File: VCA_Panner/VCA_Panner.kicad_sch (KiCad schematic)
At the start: 40 parts, among them J1 CV1, J2 Ch1_in, J3 Ch1_out, J4 CV2, J5 Ch2_in, J6 Ch2_out, SW1 SW_DPDT_x2, SW2 SW_DPDT_x2, U1 TL074, U2 AS3360, U3 TL072

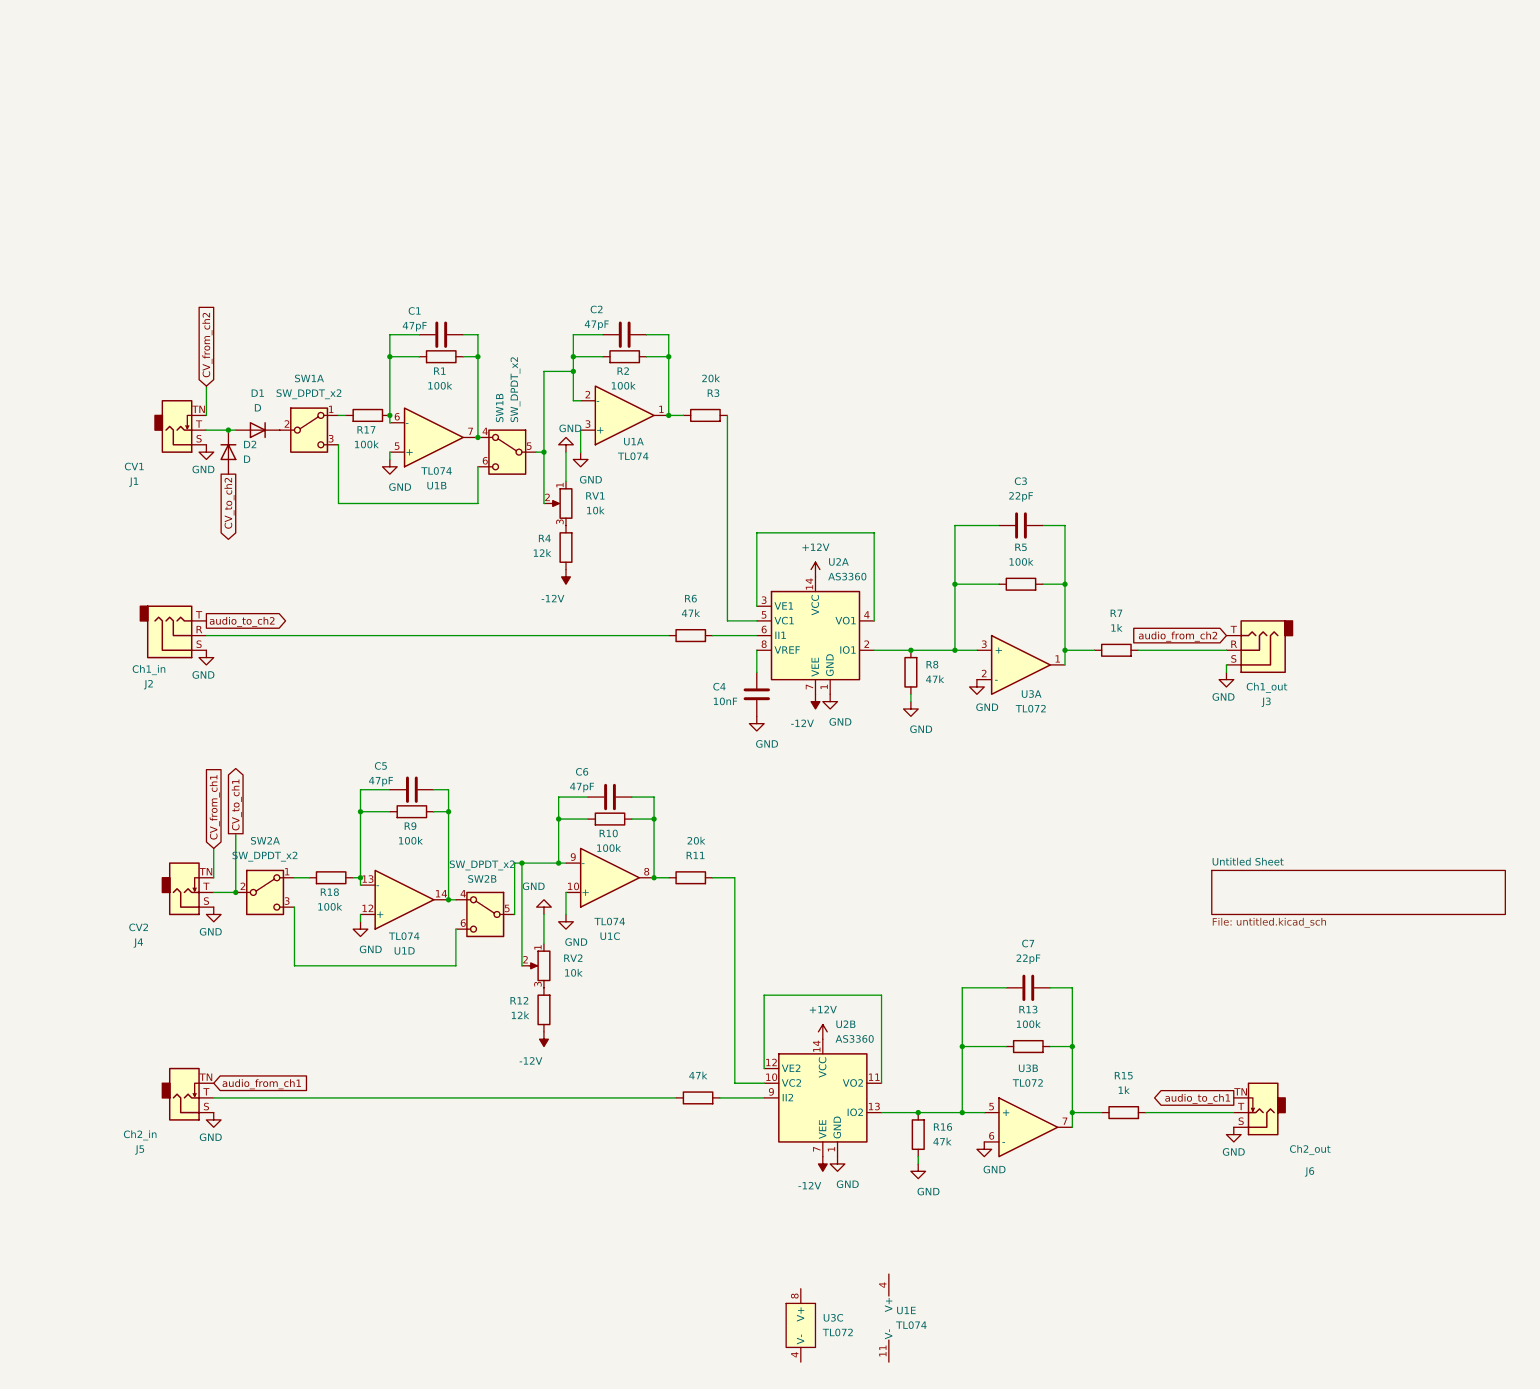
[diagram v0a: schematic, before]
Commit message: almost working
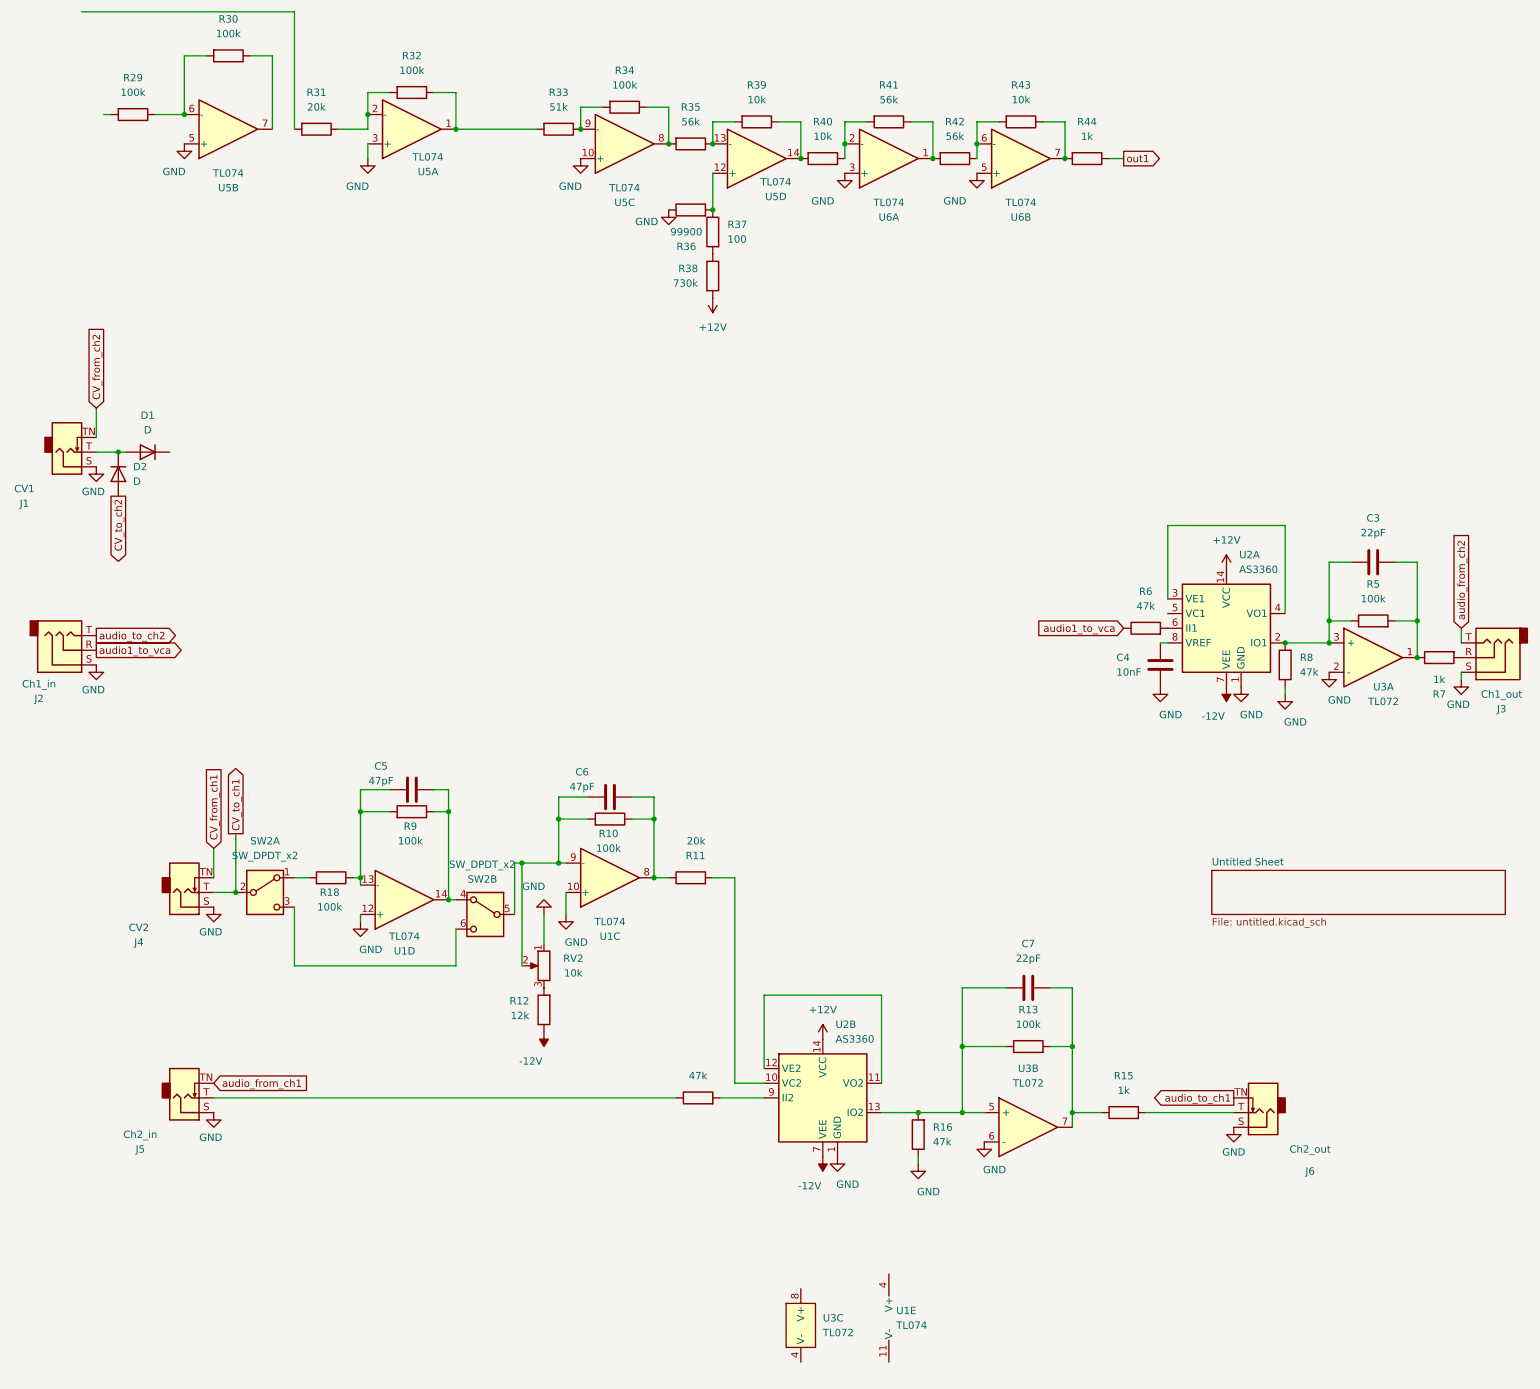
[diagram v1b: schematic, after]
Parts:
- removed C1, C2: 47pF, symbol Device:C
- removed R1, R17, R2: 100k, symbol Device:R
- removed R3: 20k, symbol Device:R
- removed R4: 12k, symbol Device:R
- removed RV1: 10k, symbol Device:R_Potentiometer
- removed SW1: SW_DPDT_x2, symbol Switch:SW_DPDT_x2
- removed unit 1 of U1
- removed unit 2 of U1
- added R29, R30, R32, R34: 100k, symbol Device:R
- added R31: 20k, symbol Device:R
- added R33: 51k, symbol Device:R
- added R35, R41, R42: 56k, symbol Device:R
- added R36: 99900, symbol Device:R
- added R37: 100, symbol Device:R
- added R38: 730k, symbol Device:R
- added R39, R40, R43: 10k, symbol Device:R
- added R44: 1k, symbol Device:R
- added U5, U6: TL074, symbol Amplifier_Operational:TL074
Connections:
- net +12V: now also R38.2
- net GND: now also R36.1, U5.10 (+), U5.3 (+), U5.5 (+), U6.3 (+), U6.5 (+)
- net audio1_to_vca: now reaches J2.R, R6.1
- new net: R32.1, R33.2, U5.1
- new net: R31.1, R32.2, U5.2 (-)
- new net: R36.2, R37.1, U5.12 (+)
- new net: R37.2, R38.1
- new net: R35.1, R39.2, U5.13 (-)
- new net: R39.1, R40.2, U5.14
- new net: R43.1, R44.2, U6.7
- new net: R42.1, R43.2, U6.6 (-)
- new net: R30.1, U5.7
- new net: R29.1, R30.2, U5.6 (-)
- new net: R33.1, R34.2, U5.9 (-)
- new net: R41.1, R42.2, U6.1
- new net: R40.1, R41.2, U6.2 (-)
- new net: R34.1, R35.2, U5.8
- new net out1: R44.1
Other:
- moved on the sheet: C3, C4, D1, D2, J1, J2, J3, R5, R6, R7, R8, U2A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

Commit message: finished schematic
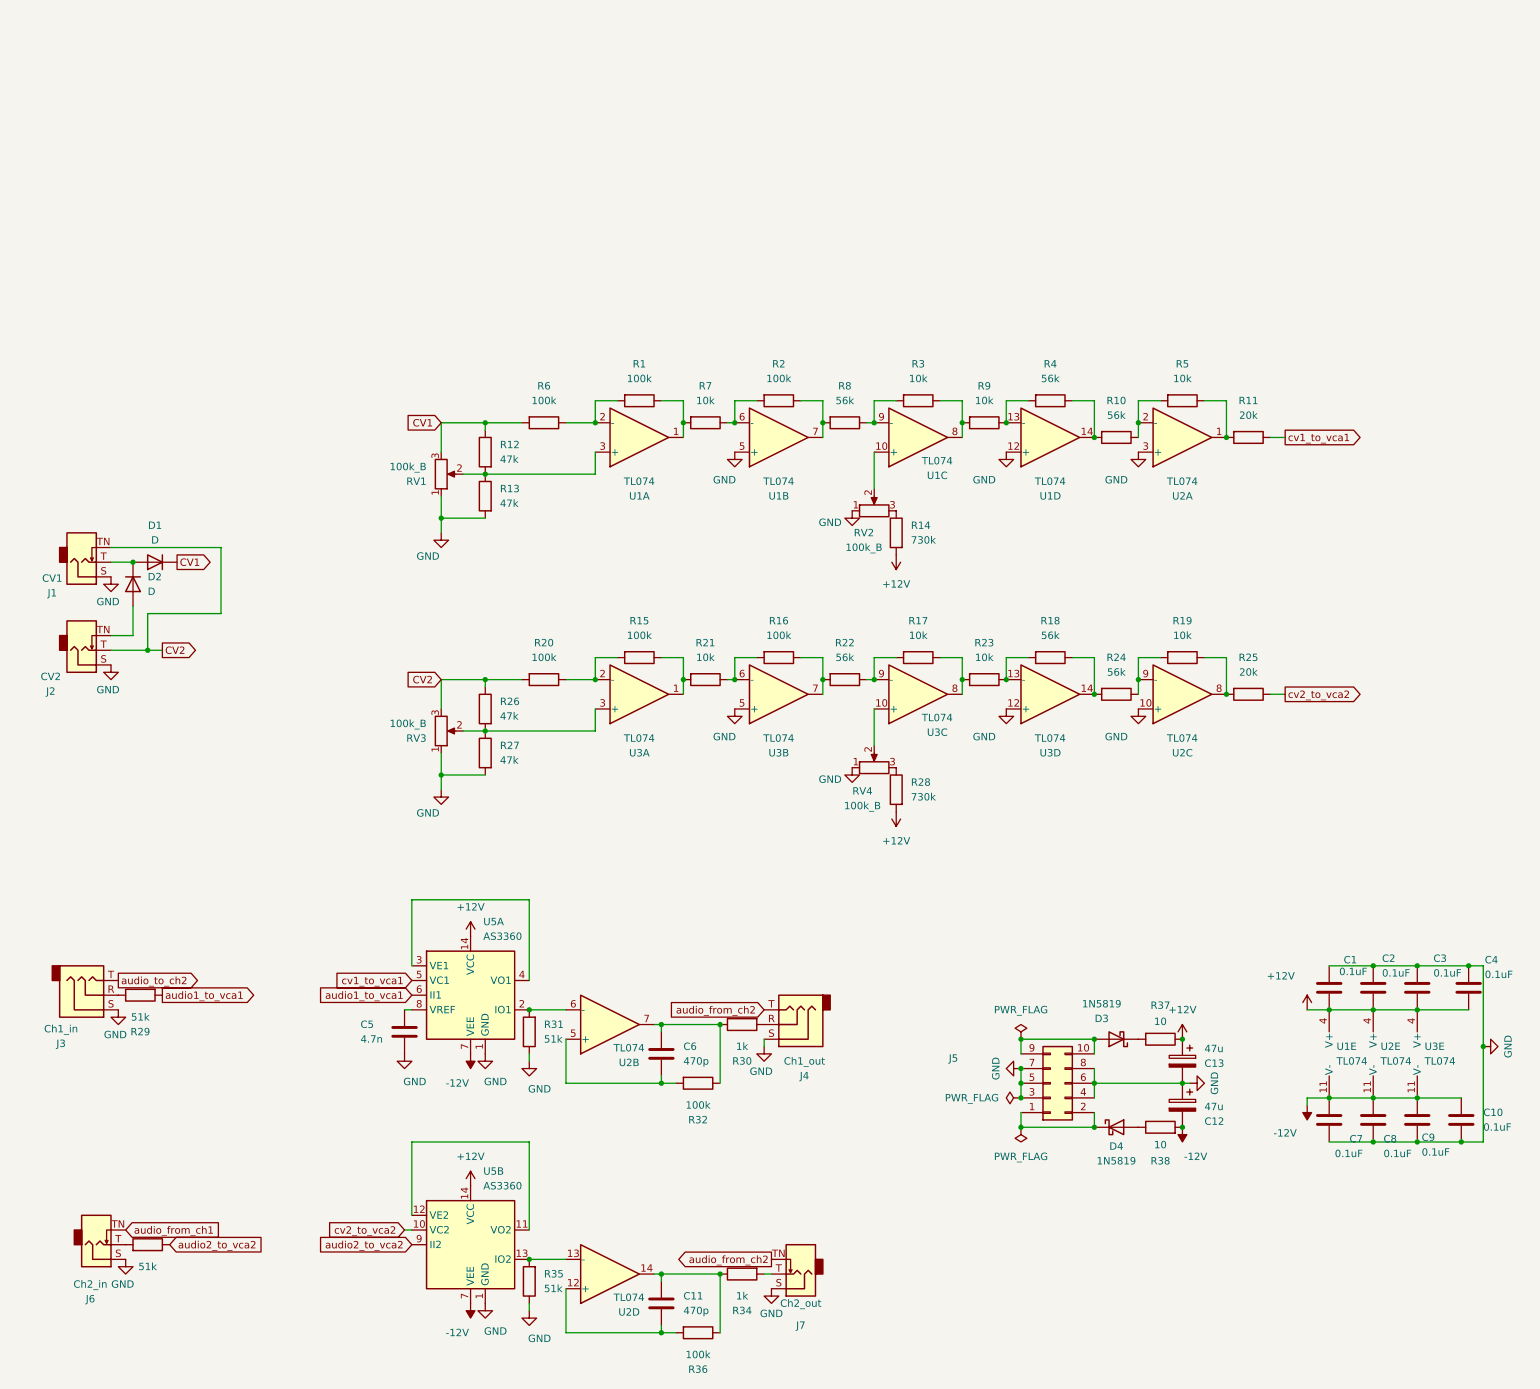
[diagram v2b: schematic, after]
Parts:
- removed C5: 47pF, symbol Device:C
- removed R30: 100k, symbol Device:R
- removed R31: 20k, symbol Device:R
- removed R39, R40, R43: 10k, symbol Device:R
- removed R41, R42: 56k, symbol Device:R
- removed R44: 1k, symbol Device:R
- removed SW2: SW_DPDT_x2, symbol Switch:SW_DPDT_x2
- removed U3: TL072, 4ms_Package_SSOP:TSSOP-8_4.4x3mm_Pitch0.65mm, symbol PCM_4ms_IC:TL072
- removed U5, U6: TL074, symbol Amplifier_Operational:TL074
- added C1, C10, C2, C4, C8, C9: 0.1uF, Capacitor_SMD:C_0805_2012Metric_Pad1.18x1.45mm_HandSolder, symbol Device:C
- added C11: 470p, Capacitor_SMD:C_0805_2012Metric_Pad1.18x1.45mm_HandSolder, symbol Device:C
- added C12, C13: 47u, Capacitor_THT:CP_Radial_D4.0mm_P2.00mm, symbol Device:C_Polarized
- added D3, D4: 1N5819, Diode_THT:D_DO-41_SOD81_P2.54mm_Vertical_AnodeUp, symbol Diode:1N5819
- added J5: ~, mort_mix:Pins_2x05_2.54mm_TH_Europower_shrouded, symbol Connector_Generic:Conn_02x05_Odd_Even
- added R1, R2, R20: 100k, Resistor_SMD:R_0805_2012Metric_Pad1.20x1.40mm_HandSolder, symbol Device:R
- added R17, R19, R21, R23, R3, R7: 10k, Resistor_SMD:R_0805_2012Metric_Pad1.20x1.40mm_HandSolder, symbol Device:R
- added R22, R24, R4, R8: 56k, Resistor_SMD:R_0805_2012Metric_Pad1.20x1.40mm_HandSolder, symbol Device:R
- added R25: 20k, Resistor_SMD:R_0805_2012Metric_Pad1.20x1.40mm_HandSolder, symbol Device:R
- added R26, R27: 47k, Resistor_SMD:R_0805_2012Metric_Pad1.20x1.40mm_HandSolder, symbol Device:R
- added R28: 730k, Resistor_SMD:R_0805_2012Metric_Pad1.20x1.40mm_HandSolder, symbol Device:R
- added RV1, RV3, RV4: 100k_B, mort_mix:Potentiometer_Alpha_RD901F-40-00D_Single_Vertical_withhole, symbol Device:R_Potentiometer
- added unit 2 of U1
- added unit 1 of U1
- added U2, U3: TL074, Package_SO:SO-14_3.9x8.65mm_P1.27mm, symbol Amplifier_Operational:TL074
- C3, C7: value 22pF -> 0.1uF; footprint (none) -> Capacitor_SMD:C_0805_2012Metric_Pad1.18x1.45mm_HandSolder
- C5: renamed from C4; value 10nF -> 4.7n; footprint (none) -> Capacitor_SMD:C_0805_2012Metric_Pad1.18x1.45mm_HandSolder
- C6: value 47pF -> 470p; footprint (none) -> Capacitor_SMD:C_0805_2012Metric_Pad1.18x1.45mm_HandSolder
- D1, D2: footprint (none) -> Diode_SMD:D_0805_2012Metric_Pad1.15x1.40mm_HandSolder
- J1: footprint (none) -> mort_mix:PJ398SM
- J2: renamed from J4; footprint (none) -> mort_mix:PJ398SM
- J3: renamed from J2; footprint (none) -> mort_mix:Jack_3.5mm_QingPu_WQP-PJ366ST_Vertical
- J4: renamed from J3; footprint (none) -> mort_mix:Jack_3.5mm_QingPu_WQP-PJ366ST_Vertical
- J6: renamed from J5; footprint (none) -> mort_mix:PJ398SM
- J7: renamed from J6; footprint (none) -> mort_mix:PJ398SM
- R10, R18: value 100k -> 56k; footprint (none) -> Resistor_SMD:R_0805_2012Metric_Pad1.20x1.40mm_HandSolder
- R11, R32, R33: footprint (none) -> Resistor_SMD:R_0805_2012Metric_Pad1.20x1.40mm_HandSolder
- R12: value 12k -> 47k; footprint (none) -> Resistor_SMD:R_0805_2012Metric_Pad1.20x1.40mm_HandSolder
- R13: value 100k -> 47k; footprint (none) -> Resistor_SMD:R_0805_2012Metric_Pad1.20x1.40mm_HandSolder
- R14: value 47k -> 730k; footprint (none) -> Resistor_SMD:R_0805_2012Metric_Pad1.20x1.40mm_HandSolder
- R15: value 1k -> 100k; footprint (none) -> Resistor_SMD:R_0805_2012Metric_Pad1.20x1.40mm_HandSolder
- R16, R6: value 47k -> 100k; footprint (none) -> Resistor_SMD:R_0805_2012Metric_Pad1.20x1.40mm_HandSolder
- R29: value 100k -> 51k; footprint (none) -> Resistor_SMD:R_0805_2012Metric_Pad1.20x1.40mm_HandSolder
- R30: renamed from R7; footprint (none) -> Resistor_SMD:R_0805_2012Metric_Pad1.20x1.40mm_HandSolder
- R31: renamed from R8; value 47k -> 51k; footprint (none) -> Resistor_SMD:R_0805_2012Metric_Pad1.20x1.40mm_HandSolder
- R34: value 100k -> 1k; footprint (none) -> Resistor_SMD:R_0805_2012Metric_Pad1.20x1.40mm_HandSolder
- R35: value 56k -> 51k; footprint (none) -> Resistor_SMD:R_0805_2012Metric_Pad1.20x1.40mm_HandSolder
- R36: value 99900 -> 100k; footprint (none) -> Resistor_SMD:R_0805_2012Metric_Pad1.20x1.40mm_HandSolder
- R37: value 100 -> 10; footprint (none) -> Resistor_SMD:R_0805_2012Metric_Pad1.20x1.40mm_HandSolder
- R38: value 730k -> 10; footprint (none) -> Resistor_SMD:R_0805_2012Metric_Pad1.20x1.40mm_HandSolder
- R5, R9: value 100k -> 10k; footprint (none) -> Resistor_SMD:R_0805_2012Metric_Pad1.20x1.40mm_HandSolder
- RV2: value 10k -> 100k_B; footprint (none) -> mort_mix:Potentiometer_Alpha_RD901F-40-00D_Single_Vertical_withhole
- U1: footprint (none) -> Package_SO:SO-14_3.9x8.65mm_P1.27mm
- U5: renamed from U2; footprint (none) -> Package_SO:SOIC-16_3.9x9.9mm_P1.27mm
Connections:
- net CV_to_ch1 is gone; now on net CV2: J2.T
- net CV_to_ch2 is gone; now on an unnamed net: D2.2 (A)
- net audio_to_ch1 is gone; now on net audio_from_ch2: J7.TN
- net +12V: now also C3.1, R14.2, R37.1, U1.4 (V+), C1.1, C13.1, C2.1, C4.2, R28.2, U2.4 (V+), U3.4 (V+); no longer R38.2
- net -12V: now also C7.2, R38.2, U1.11 (V-), C10.2, C12.2, C8.2, C9.2, U2.11 (V-), U3.11 (V-); no longer R12.1
- net GND: now also C3.2, C7.1, R13.2, R35.1, C1.2, C10.1, C12.1, C13.2, C2.2, C4.1, C8.1, C9.1, J5.3 (Pin_3), J5.4 (Pin_4), J5.5 (Pin_5), J5.6 (Pin_6), J5.7 (Pin_7), J5.8 (Pin_8), R27.2, RV1.1, RV3.1, RV4.1, U1.5 (+), U2.10 (+), U2.3 (+), U3.12 (+), U3.5 (+); no longer R16.1, R36.1, U1.10 (+)
- net at R32.1: now also C6.2, R30.1, U2.7; no longer R33.2
- net at R32.2: now also C6.1, U2.5 (+)
- net at R36.2: now also C11.1, U2.12 (+); no longer R37.1
- net at R38.1: now also D4.2 (A); no longer R37.2
- net at R31.2, U5.2 (IO1): now also U2.6 (-); no longer C3.1, R5.1
- net CV1: now reaches D1.1 (K)
- net CV1: now also R12.1, R6.2, RV1.3
- net at R12.2: now also R13.1, RV1.2, U1.3 (+); no longer RV2.3
- net at R18.2: now also R23.1, U3.13 (-)
- net at R14.1: now also RV2.3; no longer J6.T
- net at R29.1: now also J3.R
- net audio1_to_vca1: now reaches U5.6 (II1)
- net audio1_to_vca1: now also R29.2; no longer R6.2
- net at R34.2: now also J7.T; no longer R33.1
- net at R11.2: now also R5.1, U2.1; no longer U5.10 (VC2)
- net at R9.1: now also U1.13 (-), R4.2; no longer U1.14
- net cv1_to_vca1: now reaches U5.5 (VC1)
- net cv1_to_vca1: now also R11.1
- net at R34.1: now also R36.1, C11.2, U2.14; no longer R35.2
- net at R15.2: now also R20.1, U3.2 (-); no longer J7.T
- net audio2_to_vca2: now reaches U5.9 (II2)
- net audio2_to_vca2: now also R33.1; no longer R14.2
- net CV_from_ch1: no longer names the net of J2.TN
- net CV_from_ch2 renamed CV2
- net CV2: now also R20.2, R26.1, RV3.3
- net audio1_to_vca: no longer names the net of R6.1
- net audio1_to_vca: now also R1.2, U1.2 (-); no longer J3.R
- new net: R3.1, R9.2, U1.8
- new net: RV2.2, U1.10 (+)
- new net: R3.2, R8.1, U1.9 (-)
- new net: R15.1, R21.2, U3.1
- new net: R26.2, R27.1, RV3.2, U3.3 (+)
- new net: R18.1, R24.2, U3.14
- new net: R10.1, R5.2, U2.2 (-)
- new net: R10.2, R4.1, U1.14
- new net: R16.1, R22.2, U3.7
- new net: R16.2, R21.1, U3.6 (-)
- new net: R19.2, R24.1, U2.9 (-)
- new net: D3.1 (K), R37.2
- new net: R28.1, RV4.3
- new net: D3.2 (A), J5.10 (Pin_10), J5.9 (Pin_9)
- new net: R1.1, R7.2, U1.1
- new net: R17.1, R23.2, U3.8
- new net: R35.2, U2.13 (-), U5.13 (IO2)
- new net: RV4.2, U3.10 (+)
- new net: R17.2, R22.1, U3.9 (-)
- new net: J6.T, R33.2
- new net: R2.1, R8.2, U1.7
- new net: R19.1, R25.2, U2.8
- new net: D4.1 (K), J5.1 (Pin_1), J5.2 (Pin_2)
- new net: R2.2, R7.1, U1.6 (-)
- new net cv2_to_vca2: R25.1, U5.10 (VC2)
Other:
- removed sheet Untitled Sheet
- moved on the sheet: C5, D1, D2, J1, J2, J3, J4, J6, J7, R30, R31, U5A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
